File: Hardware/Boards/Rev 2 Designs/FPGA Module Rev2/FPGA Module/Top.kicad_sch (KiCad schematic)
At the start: 6 parts

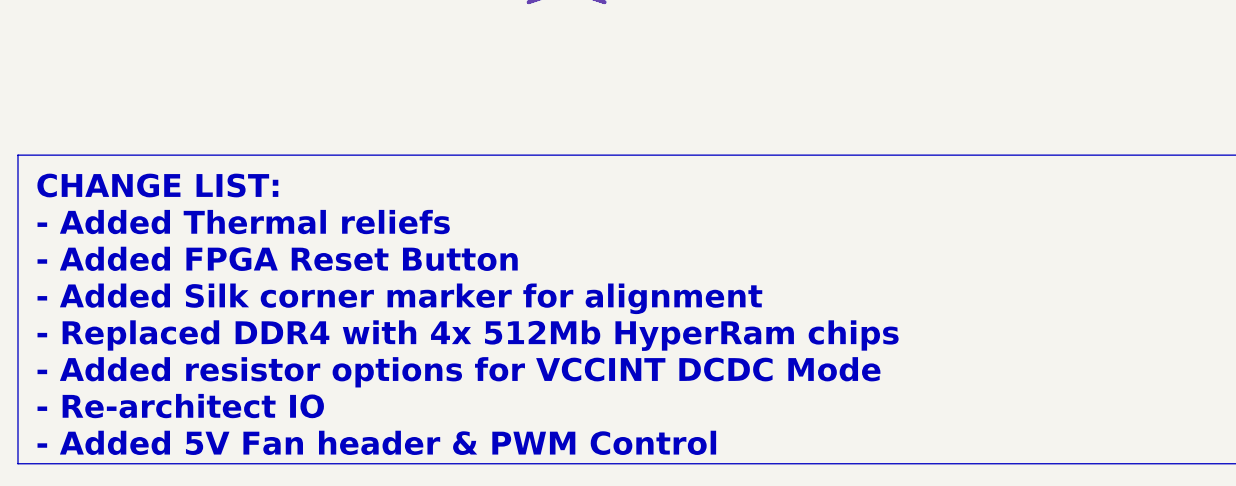
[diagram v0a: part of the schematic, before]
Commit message: Added diagrams, papers and presentations
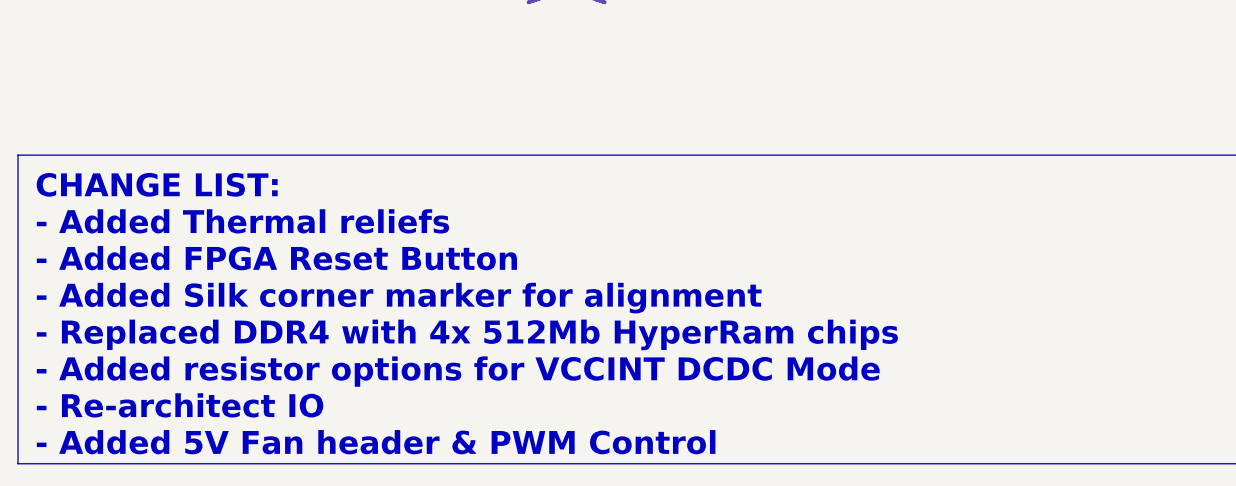
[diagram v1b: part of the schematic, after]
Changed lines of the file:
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@@
 (kicad_sch
-	(version 20231120)
+	(version 20250114)
 	(generator "eeschema")
-	(generator_version "8.0")
+	(generator_version "9.0")
 	(paper "A3")
 	(title_block
@@
 		(comment 1 "Designed by John Hofmeyr")
 	)
+	(text_box "CHANGE LIST:\n- Added Thermal reliefs\n- Added FPGA Reset Button\n- Added Silk corner marker for alignment\n- Replaced DDR4 with 4x 512Mb HyperRam chips\n- Added resistor options for VCCINT DCDC Mode\n- Re-architect IO\n- Added 5V Fan header & PWM Control\n"
+		(exclude_from_sim no)
+		(at 17.78 247.015 0)
+		(size 142.24 34.29)
+		(margins 1.905 1.905 1.905 1.905)
+		(stroke
+			(width 0)
+			(type default)
+		)
+		(fill
+			(type none)
+		)
+		(effects
+			(font
+				(size 2.54 2.54)
+				(thickness 0.508)
+				(bold yes)
+			)
+			(justify left top)
+		)
+	)
 	(junction
 		(at 201.93 180.34)
@@
 		)
 	)
-	(text_box "CHANGE LIST:\n- Added Thermal reliefs\n- Added FPGA Reset Button\n- Added Silk corner marker for alignment\n- Replaced DDR4 with 4x 512Mb HyperRam chips\n- Added resistor options for VCCINT DCDC Mode\n- Re-architect IO\n- Added 5V Fan header & PWM Control\n"
-		(exclude_from_sim no)
-		(at 17.78 247.015 0)
-		(size 142.24 34.29)
-		(stroke
-			(width 0)
-			(type default)
-		)
-		(fill
-			(type none)
-		)
-		(effects
-			(font
-				(size 2.54 2.54)
-				(thickness 0.508)
-				(bold yes)
-			)
-			(justify left top)
-		)
-	)
 	(label "SYS_SPI_MOSI"
 		(at 78.74 134.62 0)
-		(fields_autoplaced yes)
 		(effects
 			(font
@@
 	(label "SYS_SPI_MISO"
 		(at 78.74 127 0)
-		(fields_autoplaced yes)
 		(effects
 			(font
@@
 	(label "SYS_SPI_MOSI"
 		(at 300.99 161.29 180)
-		(fields_autoplaced yes)
 		(effects
 			(font
@@
 	(label "SYS_SPI_CS"
 		(at 78.74 129.54 0)
-		(fields_autoplaced yes)
 		(effects
 			(font
@@
 	(label "SYS_SPI_SCK"
 		(at 78.74 132.08 0)
-		(fields_autoplaced yes)
 		(effects
 			(font
@@
 	(label "SYS_SPI_MISO"
 		(at 300.99 153.67 180)
-		(fields_autoplaced yes)
 		(effects
 			(font
@@
 	(label "SYS_SPI_CS"
 		(at 300.99 156.21 180)
-		(fields_autoplaced yes)
 		(effects
 			(font
@@
 	(label "SYS_SPI_SCK"
 		(at 300.99 158.75 180)
-		(fields_autoplaced yes)
 		(effects
 			(font
@@
 		(at 237.49 197.485)
 		(size 44.45 15.24)
+		(exclude_from_sim no)
+		(in_bom yes)
+		(on_board yes)
+		(dnp no)
 		(fields_autoplaced yes)
 		(stroke
@@
 		(at 109.22 22.225)
 		(size 31.75 38.735)
+		(exclude_from_sim no)
+		(in_bom yes)
+		(on_board yes)
+		(dnp no)
 		(fields_autoplaced yes)
 		(stroke
@@
 		(at 302.26 30.48)
 		(size 29.21 81.28)
+		(exclude_from_sim no)
+		(in_bom yes)
+		(on_board yes)
+		(dnp no)
 		(fields_autoplaced yes)
 		(stroke
@@
 		(at 237.49 30.48)
 		(size 44.45 159.385)
+		(exclude_from_sim no)
+		(in_bom yes)
+		(on_board yes)
+		(dnp no)
 		(fields_autoplaced yes)
 		(stroke
@@
 		(at 97.79 67.31)
 		(size 43.18 80.01)
+		(exclude_from_sim no)
+		(in_bom yes)
+		(on_board yes)
+		(dnp no)
 		(fields_autoplaced yes)
 		(stroke
@@
 		(at 156.21 30.48)
 		(size 36.83 180.975)
+		(exclude_from_sim no)
+		(in_bom yes)
+		(on_board yes)
+		(dnp no)
 		(fields_autoplaced yes)
 		(stroke
@@
 		(at 309.88 201.93)
 		(size 20.955 12.065)
+		(exclude_from_sim no)
+		(in_bom yes)
+		(on_board yes)
+		(dnp no)
 		(fields_autoplaced yes)
 		(stroke
